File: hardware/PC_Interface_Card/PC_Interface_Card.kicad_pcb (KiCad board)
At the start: 2 copper layers, 146.3 x 70.7 mm, 85 parts, among them J1 GSB1C41110SSHR, J2 DM3BT-DSF-PEJS, J3 BM11B-GHS-TBT, SW1 CherryMX, SW2 CherryMX, SW3 CherryMX, SW4 CherryMX, SW5 CherryMX, SW6 TL1240YQ2JBLK, SW7 TL1240YQ2JBLK, SW8 TL1240YQ2JBLK, U1 USBLC6-2SC6, U2 TLV1117LV33DCYR, U3 MB85RS4MTYPN-GS-AWEWE1, U4 ESP32-S3-WROOM-1

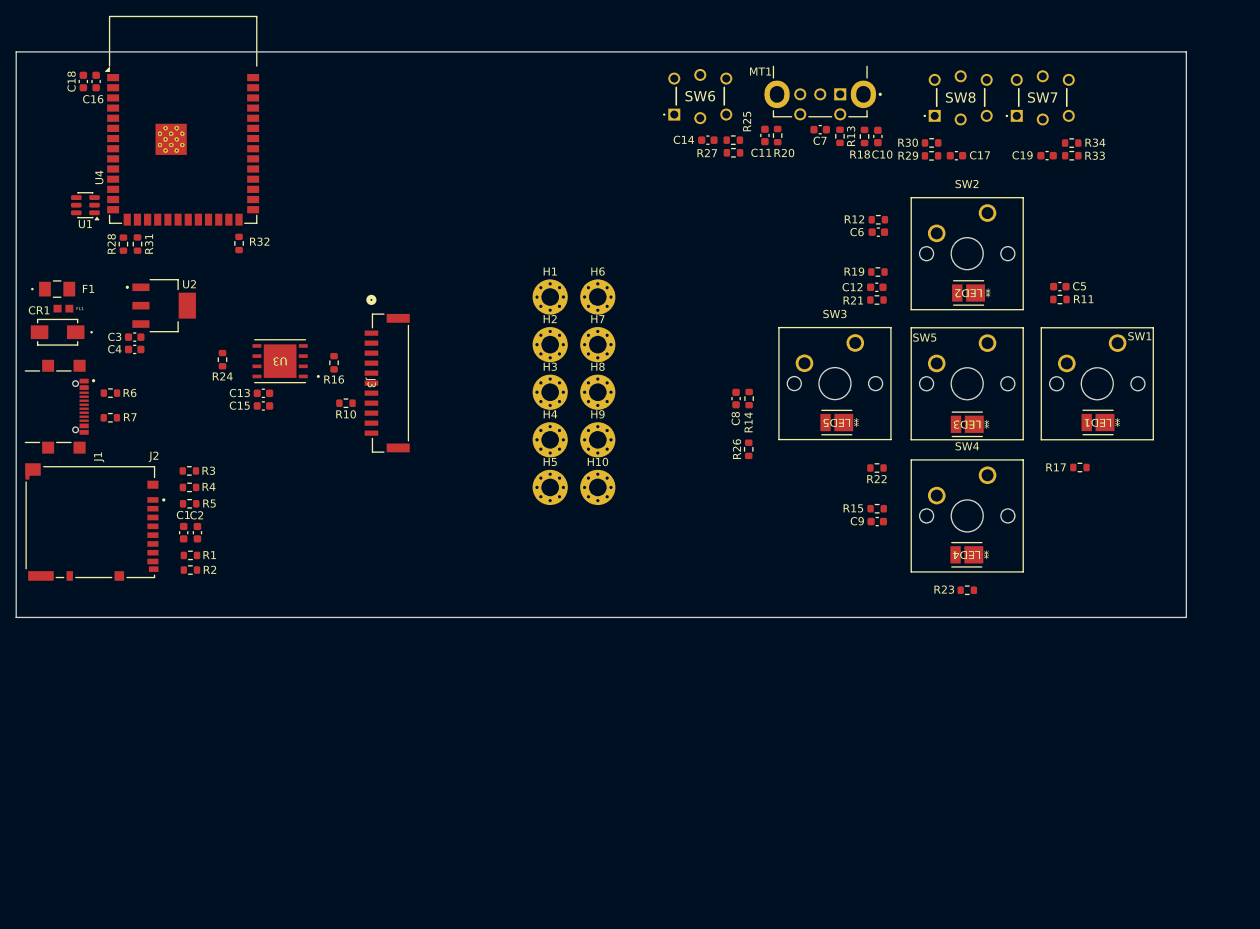
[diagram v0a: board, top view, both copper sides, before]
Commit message: Alignment of moounting holes and final layout
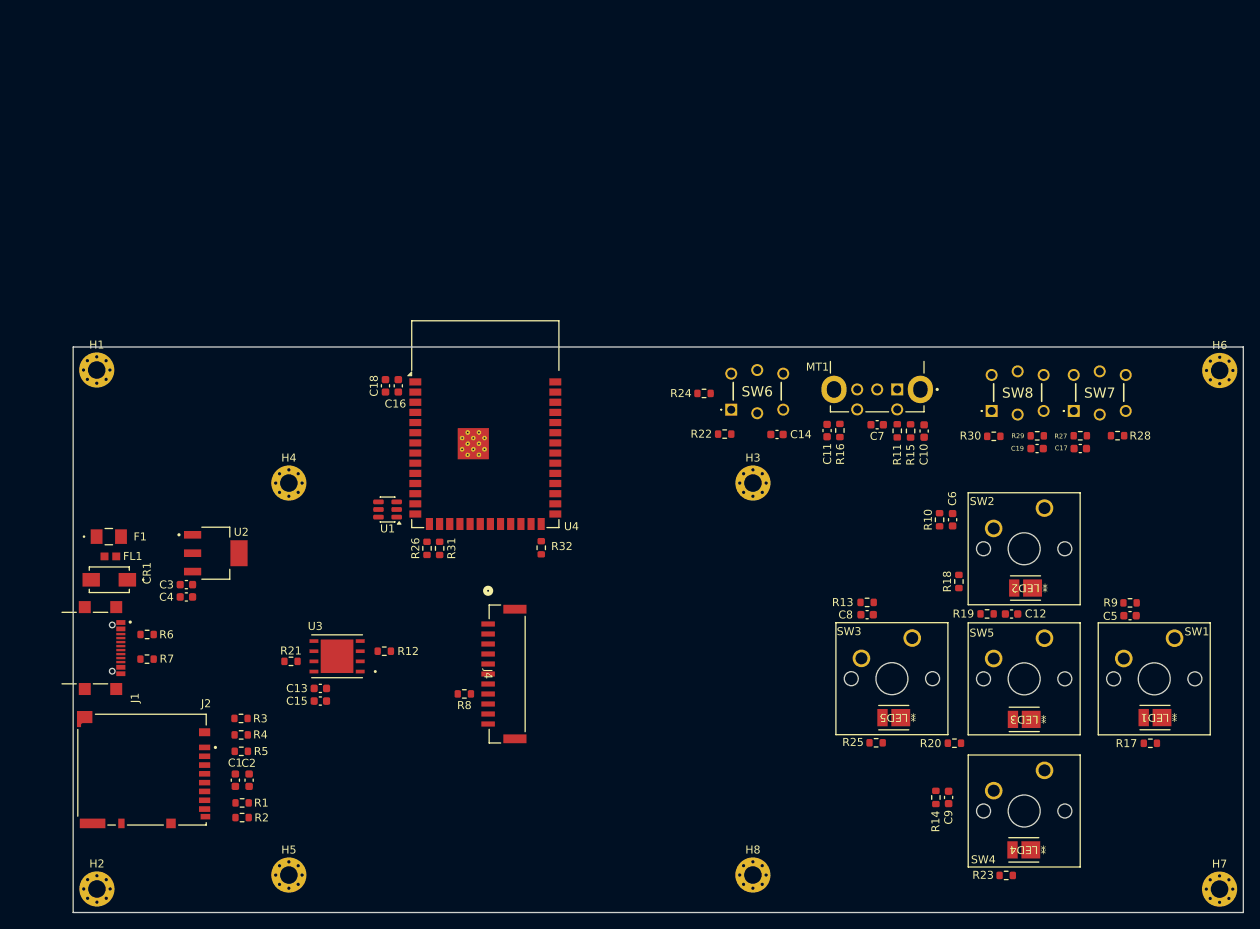
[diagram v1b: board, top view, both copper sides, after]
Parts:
- removed H10, H9: MountingHole_Pad, MountingHole:MountingHole_2.2mm_M2_Pad_Via
- removed J3: BM11B-GHS-TBT, Footprint_Project_PC_Interface:CONN11_BM11B-GHS-TBTLFSNN_JST
- removed R33: 10k_0.2W_0603, Resistor_SMD:R_0603_1608Metric
- removed R34: 68R_0.2W_0603, Resistor_SMD:R_0603_1608Metric
- added J4: BM11B-GHS-TBT, Footprint_Project_PC_Interface:CONN11_BM11B-GHS-TBTLFSNN_JST, F.Cu at (70.6, 76.0)
- added R8: 10k_0.2W_0603, Resistor_SMD:R_0603_1608Metric, F.Cu at (65.3, 78.5)
- added R9: 10k_0.2W_0603, Resistor_SMD:R_0603_1608Metric, F.Cu at (148.5, 67.1)
- R18, R20, R25: value 10k_0.2W_0603 -> 33R_0.2W_0603
- R19, R22, R26: value 33R_0.2W_0603 -> 10k_0.2W_0603
- R24, R28: value 10k_0.2W_0603 -> 68R_0.2W_0603
- R27: value 68R_0.2W_0603 -> 10k_0.2W_0603
- moved R28 126.6 mm to (146.9, 46.2), turned to 180 degrees
- moved H7 103.3 mm to (159.7, 102.9)
- moved H2 88.5 mm to (19.4, 102.9)
- moved R21 86.1 mm to (43.6, 74.4), turned to 0 degrees
- moved R12 82.0 mm to (55.3, 73.2), turned to 0 degrees
- moved R20 79.1 mm to (126.6, 84.7), turned to 180 degrees
- moved H6 78.3 mm to (159.7, 38.1)
- moved R25 77.4 mm to (116.8, 84.6), turned to 180 degrees
- moved R10 75.6 mm to (124.7, 56.7), turned to 90 degrees
- moved R16 63.8 mm to (112.2, 45.6)
- moved H8 63.4 mm to (101.4, 101.1)
- moved R24 60.3 mm to (95.3, 40.9), turned to 180 degrees
- moved H5 58.4 mm to (43.4, 101.1)
- moved R13 58.4 mm to (115.6, 67.1), turned to 0 degrees
- moved H1 57.4 mm to (19.3, 38.0)
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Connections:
- R10 pad 1: RST_DISP -> SW_UP
- R11 pad 1: SW_LEFT -> ENC_SW
- R12 pad 1: SW_UP -> Net-(U3-*WP)
- R13 pad 1: ENC_SW -> SW_RIGHT
- R13 pad 2: unconnected-(R13-Pad2) -> 3V3
- R14 pad 1: SW_RIGHT -> SW_DN
- R15 pad 1: SW_DN -> ENC_A
- R16 pad 1: Net-(U3-*WP) -> ENC_B
- R18 pad 1: ENC_A -> Net-(LED2-Pad2)
- R18 pad 2: unconnected-(R18-Pad2) -> 3V3
- R19 pad 1: Net-(LED2-Pad2) -> SW_MENU
- R20 pad 1: ENC_B -> Net-(LED3-Pad2)
- R20 pad 2: unconnected-(R20-Pad2) -> 3V3
- R21 pad 1: SW_MENU -> GND
- R21 pad 2: 3V3 -> Net-(U3-*RESET)
- R22 pad 1: Net-(LED3-Pad2) -> SW_PLAY
- R24 pad 1: GND -> Net-(SW6-+)
- R24 pad 2: Net-(U3-*RESET) -> 3V3
- R25 pad 1: SW_PLAY -> Net-(LED5-Pad2)
- R26 pad 1: Net-(LED5-Pad2) -> GND
- R26 pad 2: 3V3 -> Net-(U4-IO3)
- R27 pad 1: Net-(SW6-+) -> SW_EN
- R28 pad 1: GND -> Net-(SW7-+)
- R28 pad 2: Net-(U4-IO3) -> 3V3
- R29 pad 1: SW_EN -> SW_BOOT
- R30 pad 1: Net-(SW7-+) -> Net-(SW8-+)
